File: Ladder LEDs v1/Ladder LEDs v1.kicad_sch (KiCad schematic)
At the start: 16 parts, among them J1 01×03 Molex Nanofit Header, J2 02×02 Molex Nanofit Header, J3 Conn_01x04_Pin

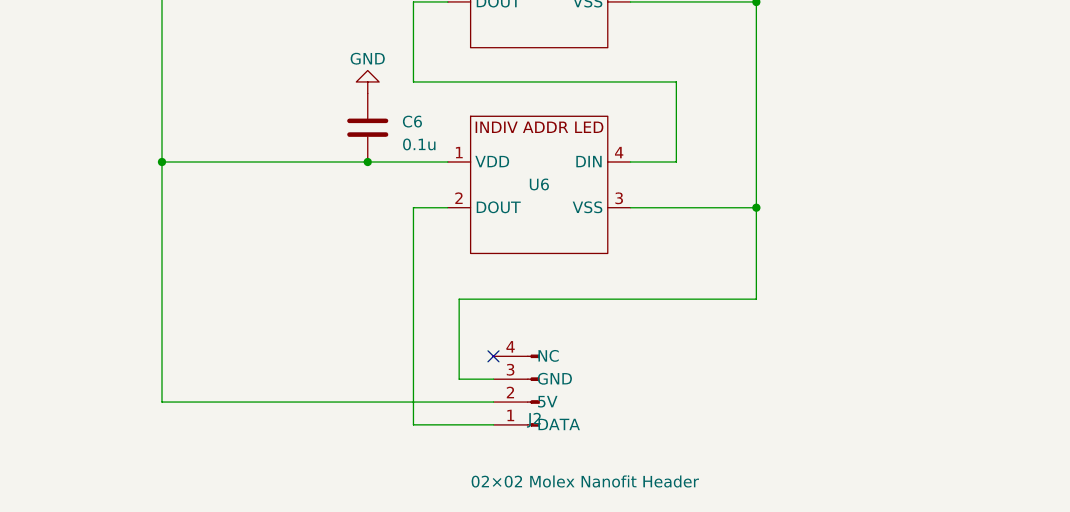
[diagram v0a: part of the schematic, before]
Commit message: Created Gerber files for OSH Park
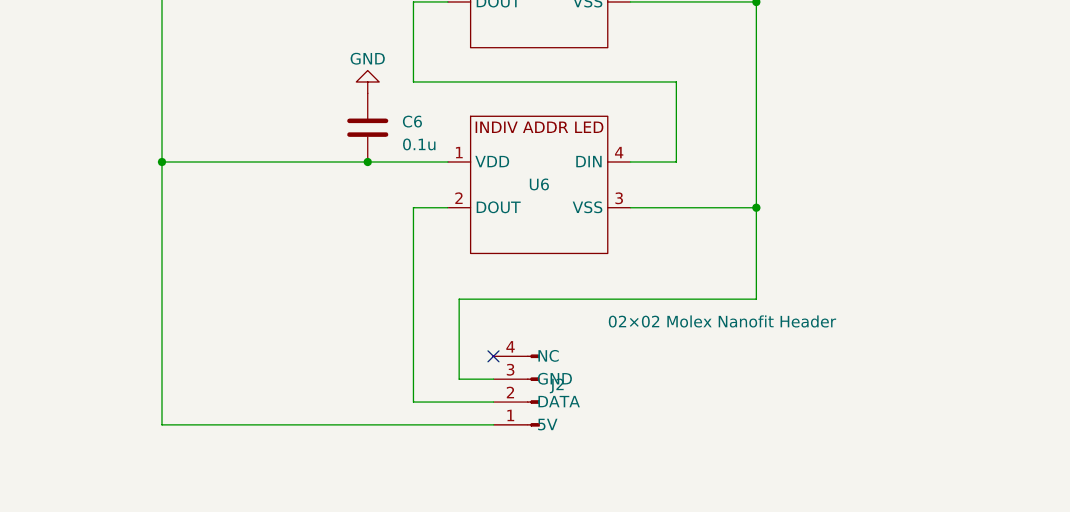
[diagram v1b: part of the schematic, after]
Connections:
- net at C1.2, C2.2, C3.2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: now also J2.1 (5V); no longer J2.2 (5V)
- net at U6.2 (DOUT): now also J2.2 (DATA); no longer J2.1 (DATA)
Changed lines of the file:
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@@
-    (stroke (width 0) (type default))
-  )
-  (wire (pts (xy 146.05 179.07) (xy 109.22 179.07))
     (stroke (width 0) (type default))
   )
@@
     (stroke (width 0) (type default))
   )
-  (wire (pts (xy 109.22 152.4) (xy 109.22 179.07))
+  (wire (pts (xy 109.22 152.4) (xy 109.22 181.61))
     (stroke (width 0) (type default))
   )
@@
     (stroke (width 0) (type default))
   )
+  (wire (pts (xy 137.16 179.07) (xy 146.05 179.07))
+    (stroke (width 0) (type default))
+  )
   (wire (pts (xy 109.22 106.68) (xy 132.08 106.68))
     (stroke (width 0) (type default))
@@
     (stroke (width 0) (type default))
   )
-  (wire (pts (xy 137.16 157.48) (xy 137.16 181.61))
-    (stroke (width 0) (type default))
-  )
   (wire (pts (xy 132.08 60.96) (xy 140.97 60.96))
     (stroke (width 0) (type default))
@@
     (stroke (width 0) (type default))
   )
+  (wire (pts (xy 109.22 181.61) (xy 146.05 181.61))
+    (stroke (width 0) (type default))
+  )
   (wire (pts (xy 137.16 66.04) (xy 137.16 74.93))
     (stroke (width 0) (type default))
@@
     (stroke (width 0) (type default))
   )
+  (wire (pts (xy 137.16 157.48) (xy 137.16 179.07))
+    (stroke (width 0) (type default))
+  )
   (wire (pts (xy 166.37 74.93) (xy 166.37 83.82))
     (stroke (width 0) (type default))
@@
   )
   (wire (pts (xy 137.16 88.9) (xy 137.16 97.79))
-    (stroke (width 0) (type default))
-  )
-  (wire (pts (xy 137.16 181.61) (xy 146.05 181.61))
     (stroke (width 0) (type default))
   )
@@
   (symbol (lib_id "Connector:Conn_01x04_Pin") (at 151.13 179.07 180) (unit 1)
     (in_bom yes) (on_board yes) (dnp no)
-    (property "Reference" "J2" (at 149.86 180.975 0)
+    (property "Reference" "J2" (at 152.4 177.165 0)
       (effects (font (size 1.27 1.27)) (justify right))
     )
-    (property "Value" "02×02 Molex Nanofit Header" (at 143.51 187.96 0)
+    (property "Value" "02×02 Molex Nanofit Header" (at 158.75 170.18 0)
       (effects (font (size 1.27 1.27)) (justify right))
     )
-    (property "Footprint" "LadderLEDLib:Molex 105405-1104" (at 151.13 179.07 0)
+    (property "Footprint" "LadderLEDLib:Molex 105405-1104" (at 149.86 187.96 0)
       (effects (font (size 1.27 1.27)) hide)
     )
@@
       (effects (font (size 1.27 1.27)) hide)
     )
-    (property "Color" "Black" (at 151.13 179.07 0)
+    (property "Color" "Black" (at 151.13 185.42 0)
       (effects (font (size 1.27 1.27)) hide)
     )
@@
       (effects (font (size 1.27 1.27)) hide)
     )
-    (property "Manufacturer" "Molex" (at 151.13 179.07 0)
-      (effects (font (size 1.27 1.27)) hide)
-    )
-    (property "URL" "https://www.digikey.com/en/products/detail/molex/1054051104/7062927?s=N4IgTCBcDaIIwAYCsAWZdEpAXQL5A" (at 151.13 179.07 0)
-      (effects (font (size 1.27 1.27)) hide)
-    )
+    (property "Manufacturer" "Molex" (at 149.86 186.69 0)
+      (effects (font (size 1.27 1.27)) hide)
+    )
+    (property "URL" "https://www.digikey.com/en/products/detail/molex/1054051104/7062927?s=N4IgTCBcDaIIwAYCsAWZdEpAXQL5A" (at 149.86 187.96 0)
+      (effects (font (size 1.27 1.27)) hide)
+    )
